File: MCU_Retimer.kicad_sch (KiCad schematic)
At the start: 36 parts, among them J10 SWD, J11 UART, J12 I2C1, Q16 AO3401A, Q17 2N7002W, U12 STM32F030C8Tx

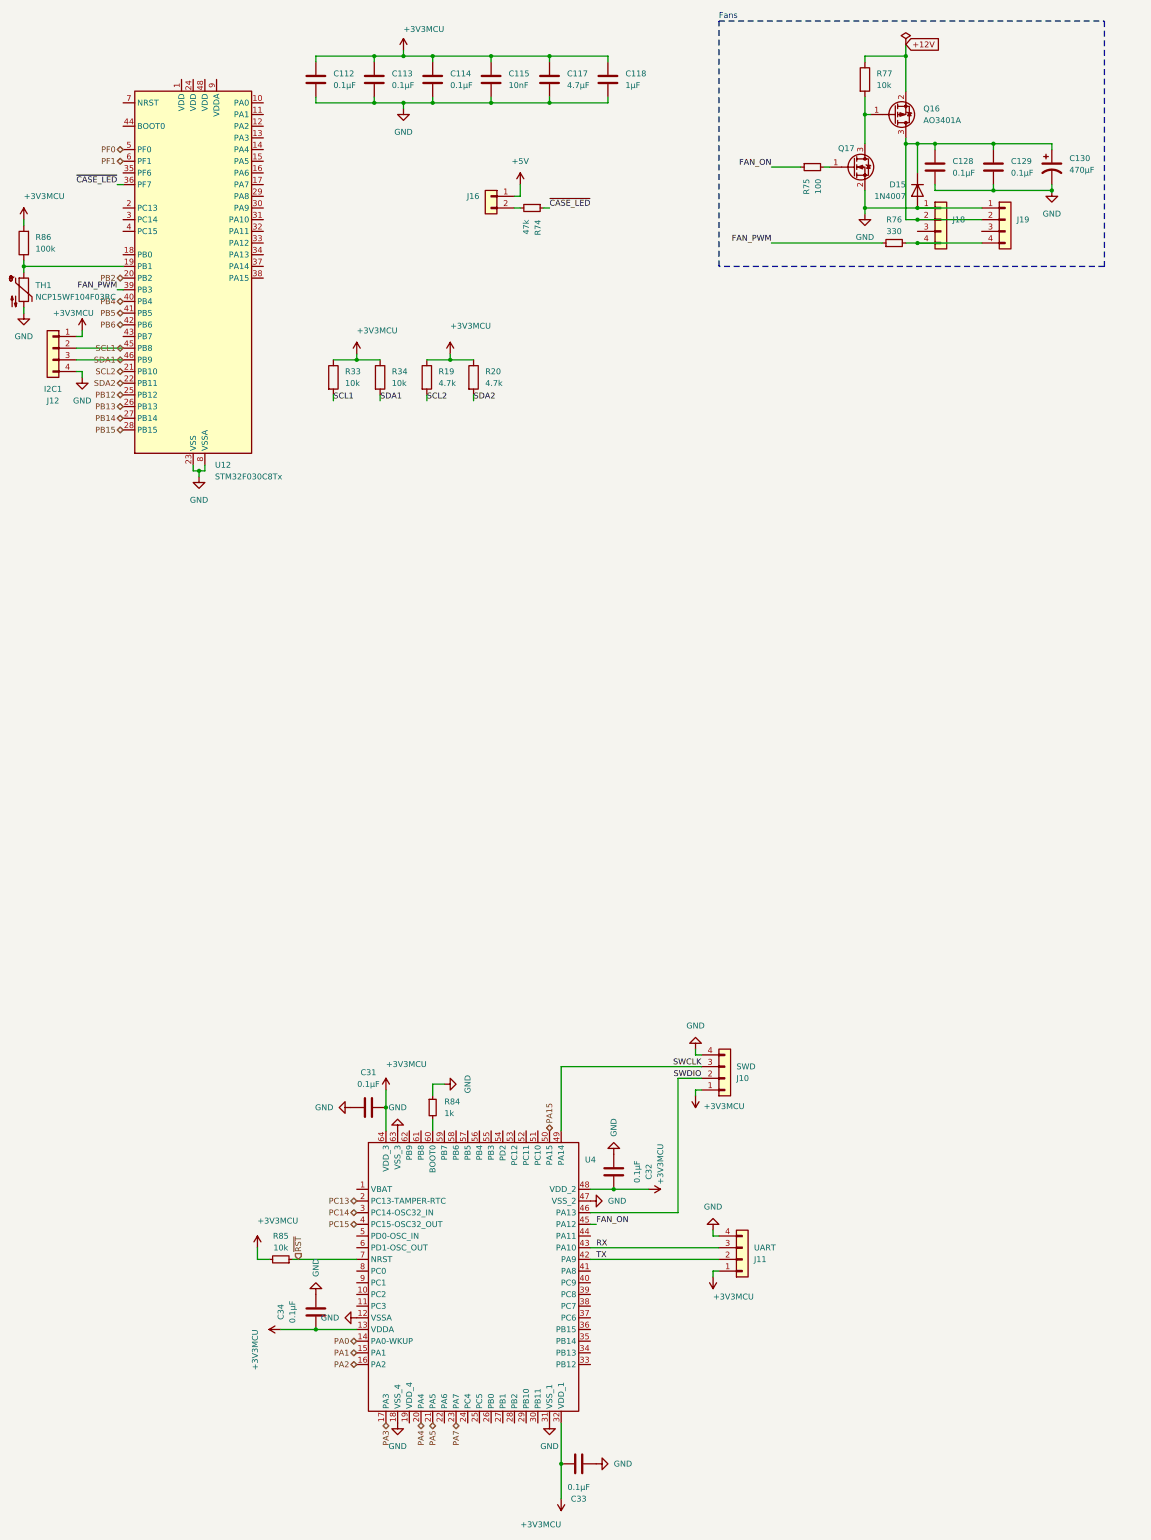
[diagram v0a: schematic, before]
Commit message: Update MCU_Retimer.kicad_sch
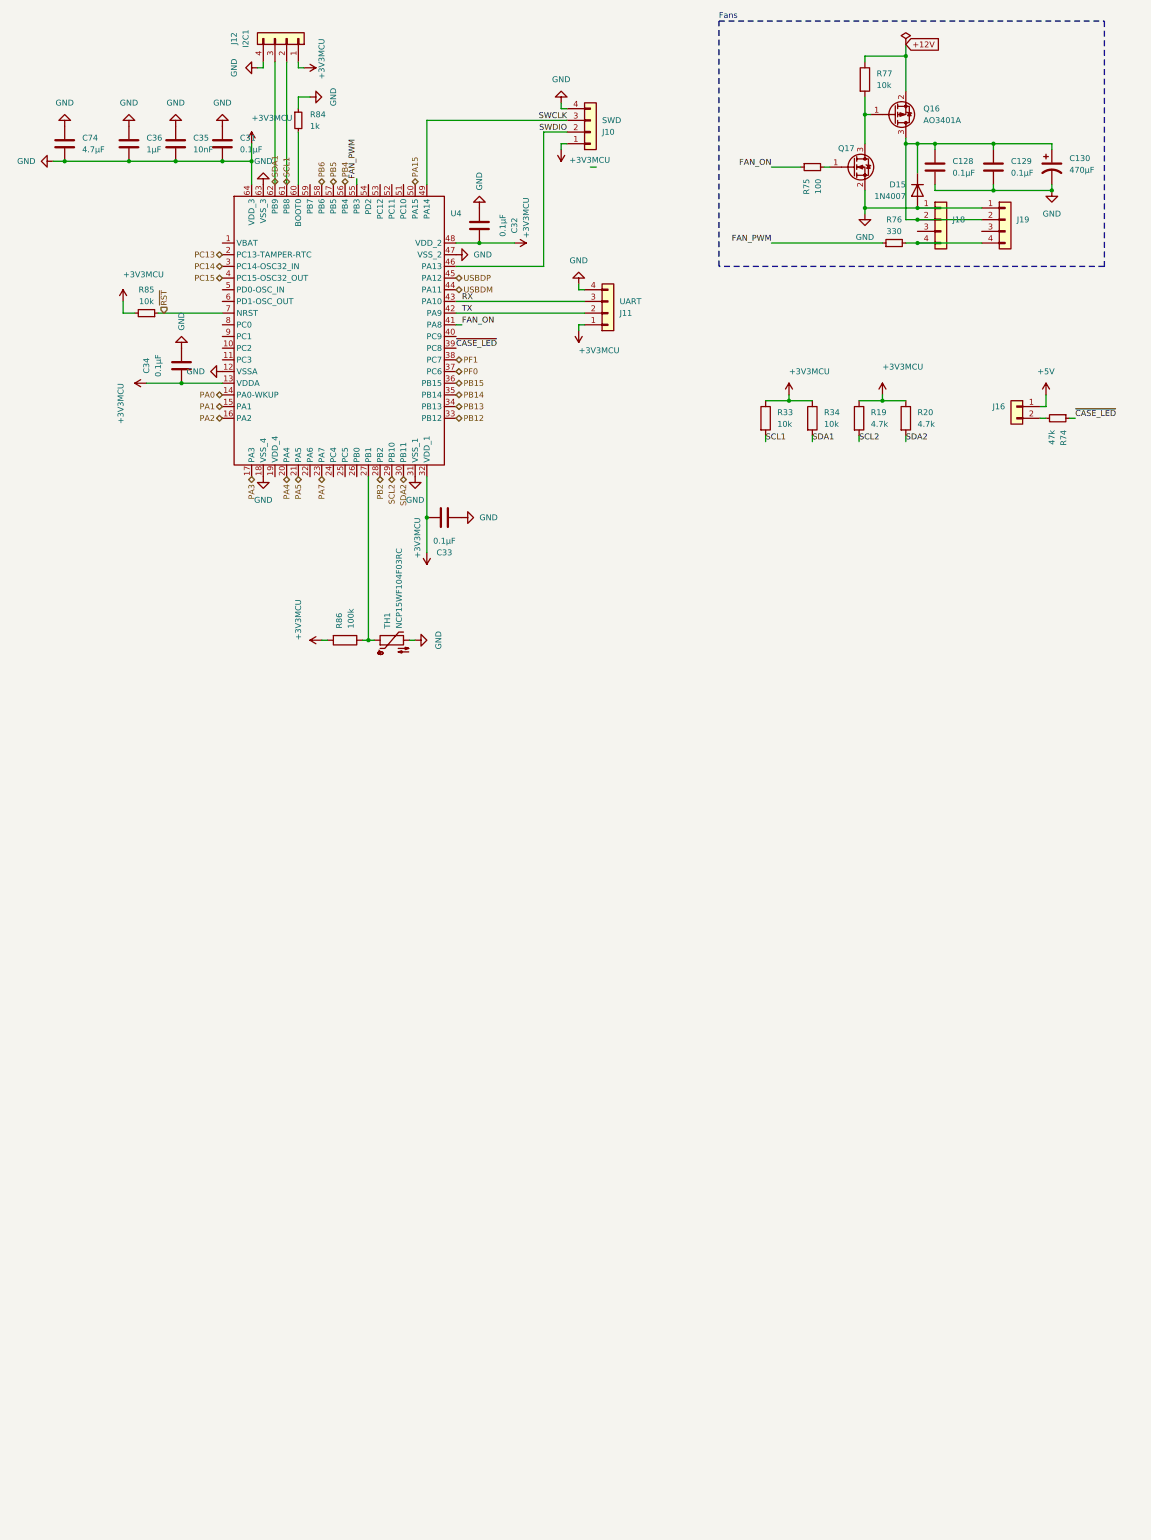
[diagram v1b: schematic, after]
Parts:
- removed C112, C113, C114: 0.1µF, Capacitor_SMD:C_0402_1005Metric, symbol Device:C
- removed C115: 10nF, Capacitor_SMD:C_0402_1005Metric, symbol Device:C
- removed C117: 4.7µF, Capacitor_SMD:C_0402_1005Metric, symbol Device:C
- removed C118: 1µF, Capacitor_SMD:C_0402_1005Metric, symbol Device:C
- removed U12: STM32F030C8Tx, Package_QFP:LQFP-48_7x7mm_P0.5mm, symbol MCU_ST_STM32F0:STM32F030C8Tx
- added C35: 10nF, Capacitor_SMD:C_0402_1005Metric, symbol Device:C
- added C36: 1µF, Capacitor_SMD:C_0402_1005Metric, symbol Device:C
- added C74: 4.7µF, Capacitor_SMD:C_0402_1005Metric, symbol Device:C
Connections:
- net GND is gone; now on net +3V3MCU: C128.2, C129.2, C130.2, C31.1, C32.1, C33.1, C34.1, D15.2 (A), J10.4 (Pin_4), J11.4 (Pin_4), J12.4 (Pin_4), J18.1 (Pin_1), J19.1 (Pin_1), Q17.2 (S), R84.1, TH1.2, U4.12 (VSSA), U4.18 (VSS_4), U4.31 (VSS_1), U4.47 (VSS_2), U4.63 (VSS_3)
- net +3V3MCU: now also C35.1, C35.2, C36.1, C36.2, C74.1, C74.2
- net FAN_ON: now also U4.41 (PA8); no longer U4.45 (PA12)
- net FAN_PWM: now also U4.55 (PB3)
- net PB12: now also U4.33 (PB12)
- net PB13: now also U4.34 (PB13)
- net PB14: now also U4.35 (PB14)
- net PB15: now also U4.36 (PB15)
- net PB2: now also U4.28 (PB2)
- net PB4: now also U4.56 (PB4)
- net PB5: now also U4.57 (PB5)
- net PB6: now also U4.58 (PB6)
- net PF0: now also U4.37 (PC6)
- net PF1: now also U4.38 (PC7)
- net SCL1: now also U4.61 (PB8)
- net SCL2: now also U4.29 (PB10)
- net SDA1: now also U4.62 (PB9)
- net SDA2: now also U4.30 (PB11)
- net ~{CASE_LED}: now also U4.39 (PC8)
- net at R86.1, TH1.1: now also U4.27 (PB1)
- net USBDM: now reaches U4.44 (PA11)
- new net USBDP: U4.45 (PA12)
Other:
- moved on the sheet: C32, C33, C34, J10, J11, J12, J16, R19, R20, R33, R34, R74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
